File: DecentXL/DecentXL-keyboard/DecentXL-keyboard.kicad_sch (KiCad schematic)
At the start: 208 parts, among them J1 Conn_02x12_Odd_Even, J2 Conn_01x26, J3 Conn_01x04, SW0 SW_Push_45deg, SW1 SW_Push_45deg, SW2 SW_Push_45deg, SW3 SW_Push_45deg, SW4 SW_Push_45deg, SW5 SW_Push_45deg, SW6 SW_Push_45deg, SW8 SW_Push_45deg, SW9 SW_Push_45deg

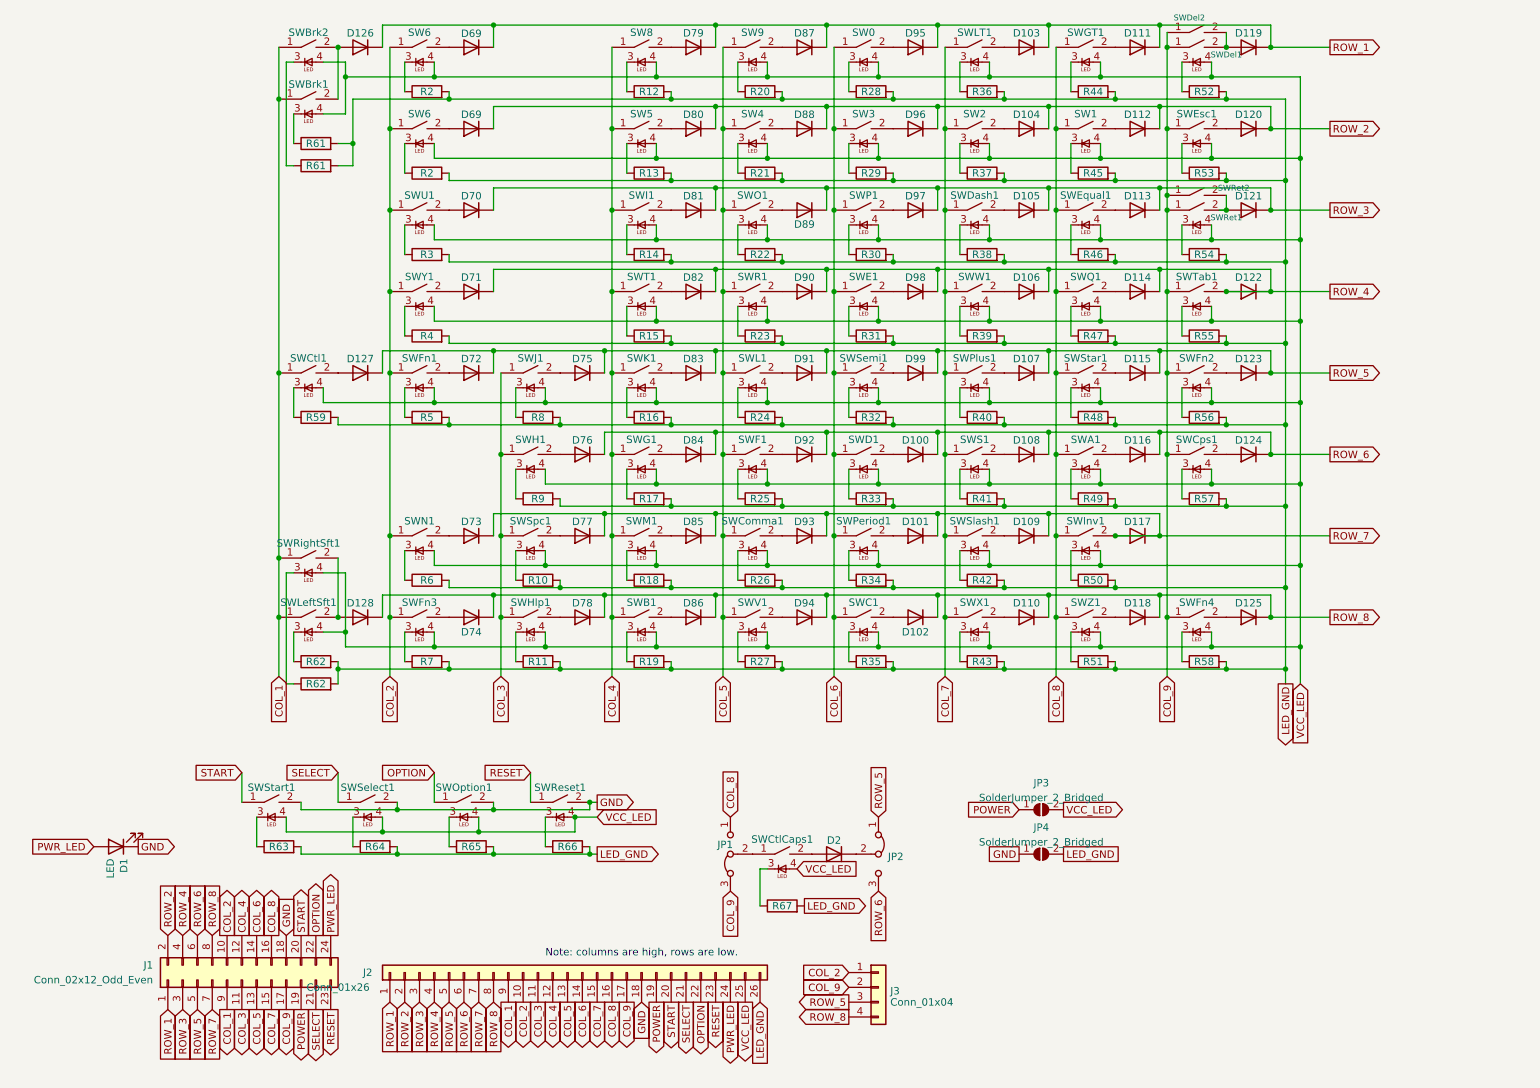
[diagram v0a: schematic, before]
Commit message: DecentXL PCB
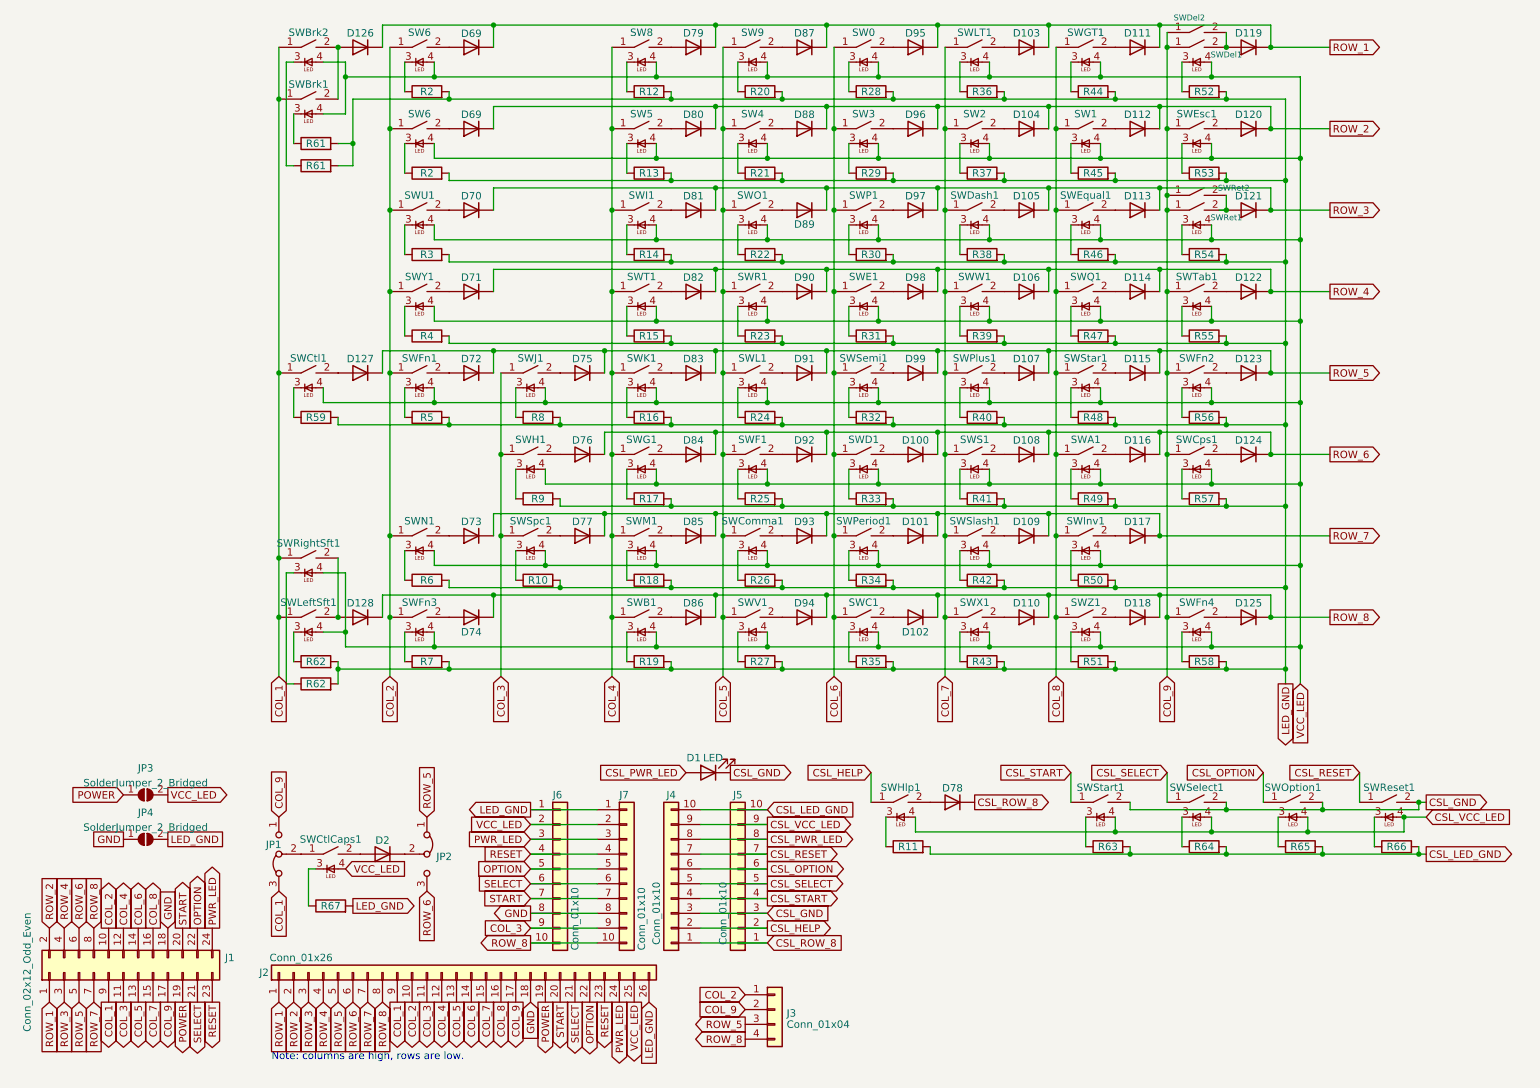
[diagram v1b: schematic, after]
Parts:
- added J4, J7: Conn_01x10, Connector_PinHeader_2.54mm:PinHeader_1x10_P2.54mm_Vertical, symbol Connector_Generic:Conn_01x10
- added J5, J6: Conn_01x10, Connector_FFC-FPC:TE_1-1734839-0_1x10-1MP_P0.5mm_Horizontal, symbol Connector_Generic:Conn_01x10
- D100, D101, D102, D103, D104, D105, D106, D107, D108, D109, D110, D111, D112, D113, D114, D115, D116, D117, D118, D119, D120, D121, D122, D123, D124, D125, D126, D127, D128, D2, D69, D70, D71, D72, D73, D74, D75, D76, D77, D78, D79, D80, D81, D82, D83, D84, D85, D86, D87, D88, D89, D90, D91, D92, D93, D94, D95, D96, D97, D98, D99: footprint Diode_SMD:D_SOD-123 -> DecentXL:D_SOD-123
- R10, R11, R12, R13, R14, R15, R16, R17, R18, R19, R2, R20, R21, R22, R23, R24, R25, R26, R27, R28, R29, R3, R30, R31, R32, R33, R34, R35, R36, R37, R38, R39, R4, R40, R41, R42, R43, R44, R45, R46, R47, R48, R49, R5, R50, R51, R52, R53, R54, R55, R56, R57, R58, R59, R6, R61, R62, R63, R64, R65, R66, R67, R7, R8, R9: footprint Resistor_SMD:R_0603_1608Metric -> DecentXL:R_0603_1608Metric
- SWBrk2: footprint DecentXL:MX-1-00U-LED -> DecentXL:MX-1-25U-LED
- SWFn1, SWFn2, SWFn3, SWFn4, SWHlp1, SWOption1, SWReset1, SWSelect1, SWStart1: footprint DecentXL:MX-1-50U-Atari-Fn-LED -> DecentXL:MX-1-00U-LED
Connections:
- net COL_1: now also JP1.3 (B)
- net COL_3: now also J6.9 (Pin_9), J7.9 (Pin_9); no longer SWHlp1.1
- net COL_8: no longer JP1.1 (A)
- net COL_9: now also JP1.1 (A); no longer JP1.3 (B)
- net GND: now also J6.8 (Pin_8), J7.8 (Pin_8); no longer D1.1 (K), SWOption1.2, SWReset1.2, SWSelect1.2, SWStart1.2
- net LED_GND: now also J6.1 (Pin_1), J7.1 (Pin_1); no longer R11.2, R63.2, R64.2, R65.2, R66.2
- net OPTION: now also J6.5 (Pin_5), J7.5 (Pin_5); no longer SWOption1.1
- net PWR_LED: now also J6.3 (Pin_3), J7.3 (Pin_3); no longer D1.2 (A)
- net RESET: now also J6.4 (Pin_4), J7.4 (Pin_4); no longer SWReset1.1
- net ROW_4: no longer D122.2 (A), SWTab1.2
- net ROW_7: no longer D117.2 (A), SWInv1.2
- net ROW_8: now also J6.10 (Pin_10), J7.10 (Pin_10); no longer D78.1 (K)
- net SELECT: now also J6.6 (Pin_6), J7.6 (Pin_6); no longer SWSelect1.1
- net START: now also J6.7 (Pin_7), J7.7 (Pin_7); no longer SWStart1.1
- net VCC_LED: now also J6.2 (Pin_2), J7.2 (Pin_2); no longer SWHlp1.4, SWOption1.4, SWReset1.4, SWSelect1.4, SWStart1.4
- new net: D122.2 (A), SWTab1.2
- new net: D117.2 (A), SWInv1.2
- new net CSL_GND: D1.1 (K), J4.3 (Pin_3), J5.3 (Pin_3), SWOption1.2, SWReset1.2, SWSelect1.2, SWStart1.2
- new net CSL_HELP: J4.2 (Pin_2), J5.2 (Pin_2), SWHlp1.1
- new net CSL_LED_GND: J4.10 (Pin_10), J5.10 (Pin_10), R11.2, R63.2, R64.2, R65.2, R66.2
- new net CSL_OPTION: J4.6 (Pin_6), J5.6 (Pin_6), SWOption1.1
- new net CSL_PWR_LED: D1.2 (A), J4.8 (Pin_8), J5.8 (Pin_8)
- new net CSL_RESET: J4.7 (Pin_7), J5.7 (Pin_7), SWReset1.1
- new net CSL_ROW_8: D78.1 (K), J4.1 (Pin_1), J5.1 (Pin_1)
- new net CSL_SELECT: J4.5 (Pin_5), J5.5 (Pin_5), SWSelect1.1
- new net CSL_START: J4.4 (Pin_4), J5.4 (Pin_4), SWStart1.1
- new net CSL_VCC_LED: J4.9 (Pin_9), J5.9 (Pin_9), SWHlp1.4, SWOption1.4, SWReset1.4, SWSelect1.4, SWStart1.4
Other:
- moved on the sheet: D1, D2, D78, J1, J2, J3, JP1, JP2, JP3, JP4, R11, R63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
